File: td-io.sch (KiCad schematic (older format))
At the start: 121 parts, among them J1 USB_A, J2 USB_B, J3 JAMMA_Edge, J4 Conn_Coaxial, J5 DB15_Female_HighDensity, J6 Conn_02x04_Top_Bottom, J7 Conn_02x17_Odd_Even, J8 Conn_Coaxial, J9 Conn_01x04_Male, Q1 FDS6930B, Q2 ZXMS6004DN8, Q3 ZXMS6004DN8, SW1 SW_DIP_x02, SW2 SW_DIP_x01, U1 TPA3138D2, U10 Pico, U11 TL081, U12 CPC1017N, U13 74LS165, U2 ISL3175EIBZ-T, U3 ADA4891-3, U4 74LS86, U5 AT24CS01-SSHM, U6 74LS165, U7 TPS568230, U8 74LS165, U9 74LS165

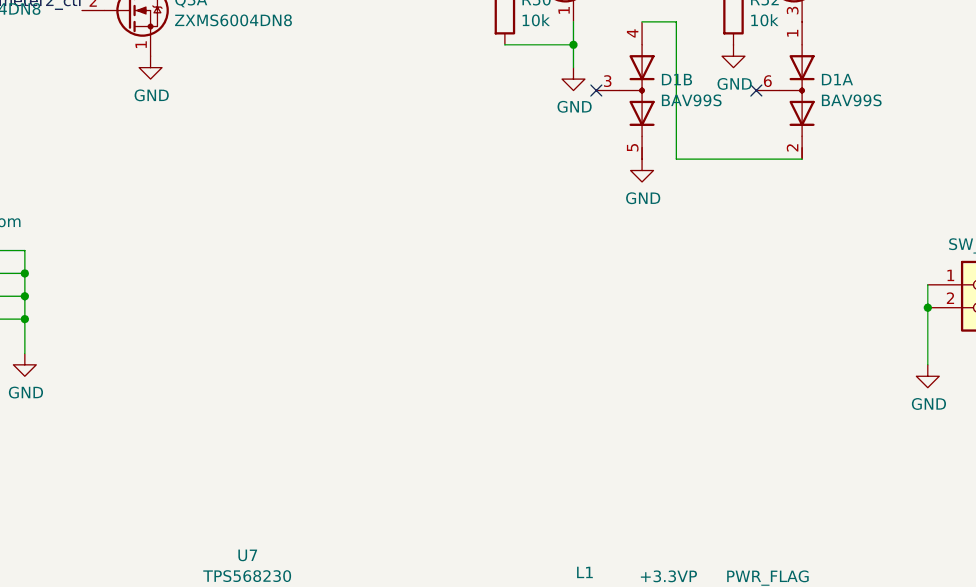
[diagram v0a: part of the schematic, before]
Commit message: Add todo
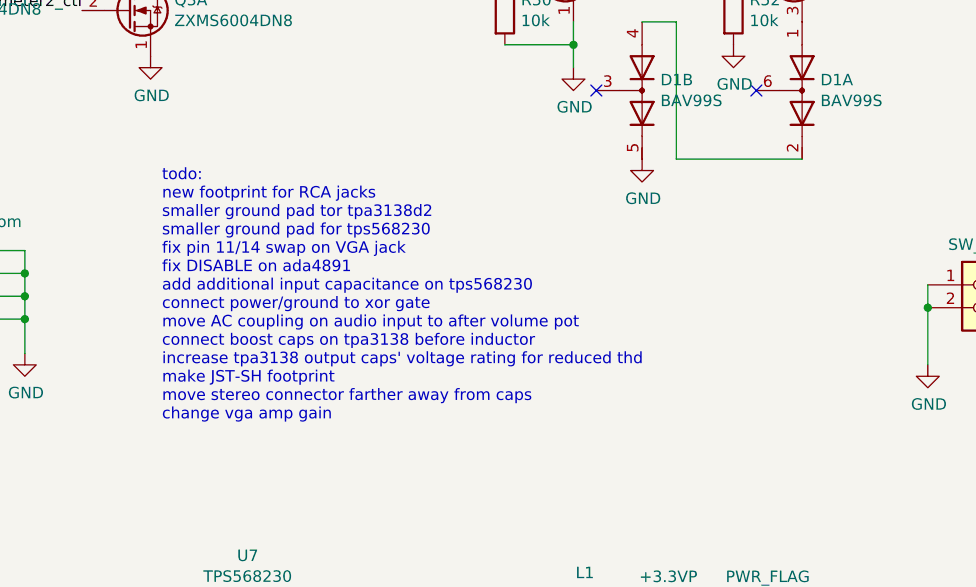
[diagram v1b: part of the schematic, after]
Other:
- note added: "todo:\nnew footprint for RCA jacks\nsmaller ground pad tor tpa3138d2\nsmaller ground pad for tps568230\nfix pin 11/14 swap on VGA jack\nfix DISABLE on ada4891\nadd additional input capacitance on tps568230\nconnect power/ground to xor gate\nmove AC coupling on audio input to after volume pot\nconnect boost caps on tpa3138 before inductor\nincrease tpa3138 output caps' voltage rating for reduced t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"
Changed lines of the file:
@@
 NoConn ~ 15450 3950
 NoConn ~ 13800 3950
+Text Notes 8700 9100 0    50   ~ 0
+todo:\nnew footprint for RCA jacks\nsmaller ground pad tor tpa3138d2\nsmaller ground pad for tps568230\nfix pin 11/14 swap on VGA jack\nfix DISABLE on ada4891\nadd additional input capacitance on tps568230\nconnect power/ground to xor gate\nmove AC coupling on audio input to after volume pot\nconnect boost caps on tpa3138 before inductor\nincrease tpa3138 output caps' voltage rating for reduced thd\nmake JST-SH footprint\nmove stereo connector farther away from caps\nchange vga amp gain
 $EndSCHEMATC
